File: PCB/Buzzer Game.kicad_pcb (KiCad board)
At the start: 2 copper layers, 50 x 50 mm, 23 parts, among them J1 Conn_01x02, Q1 BC547, Q2 BC547, U1 74LS373

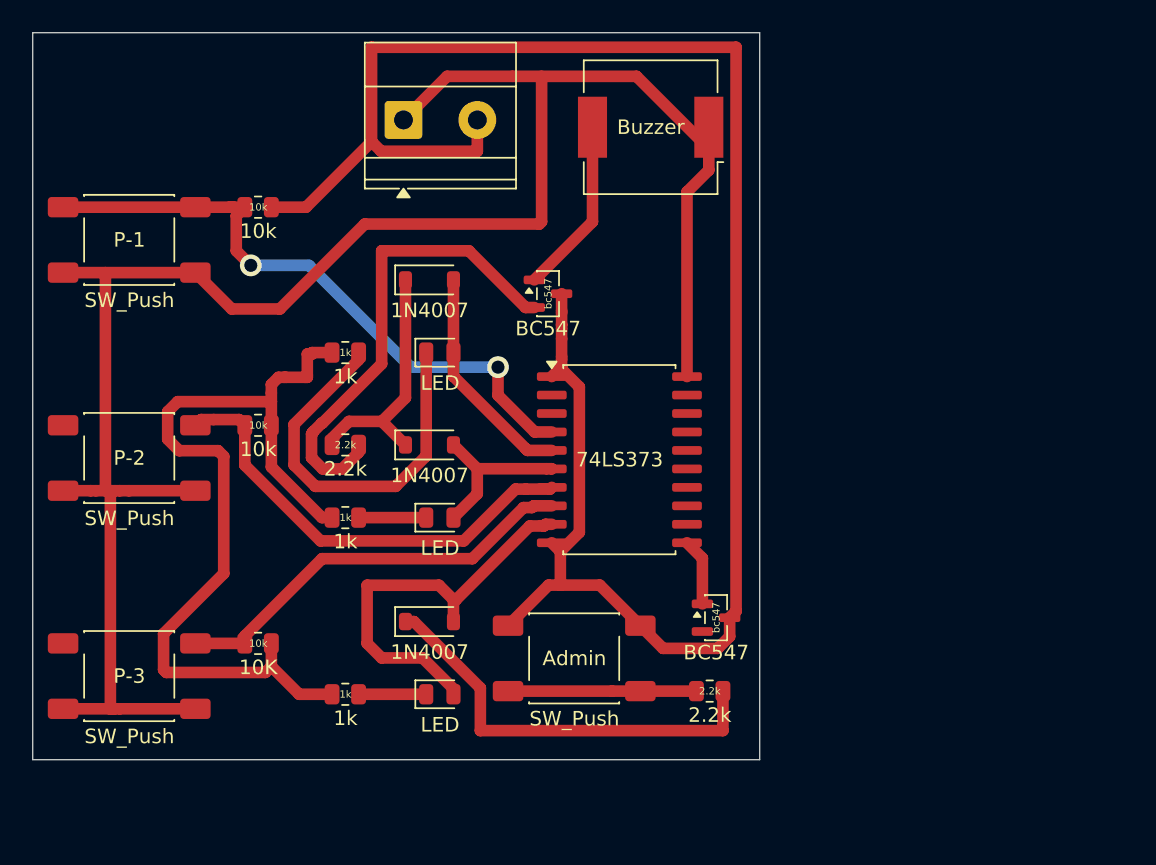
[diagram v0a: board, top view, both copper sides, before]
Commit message: .
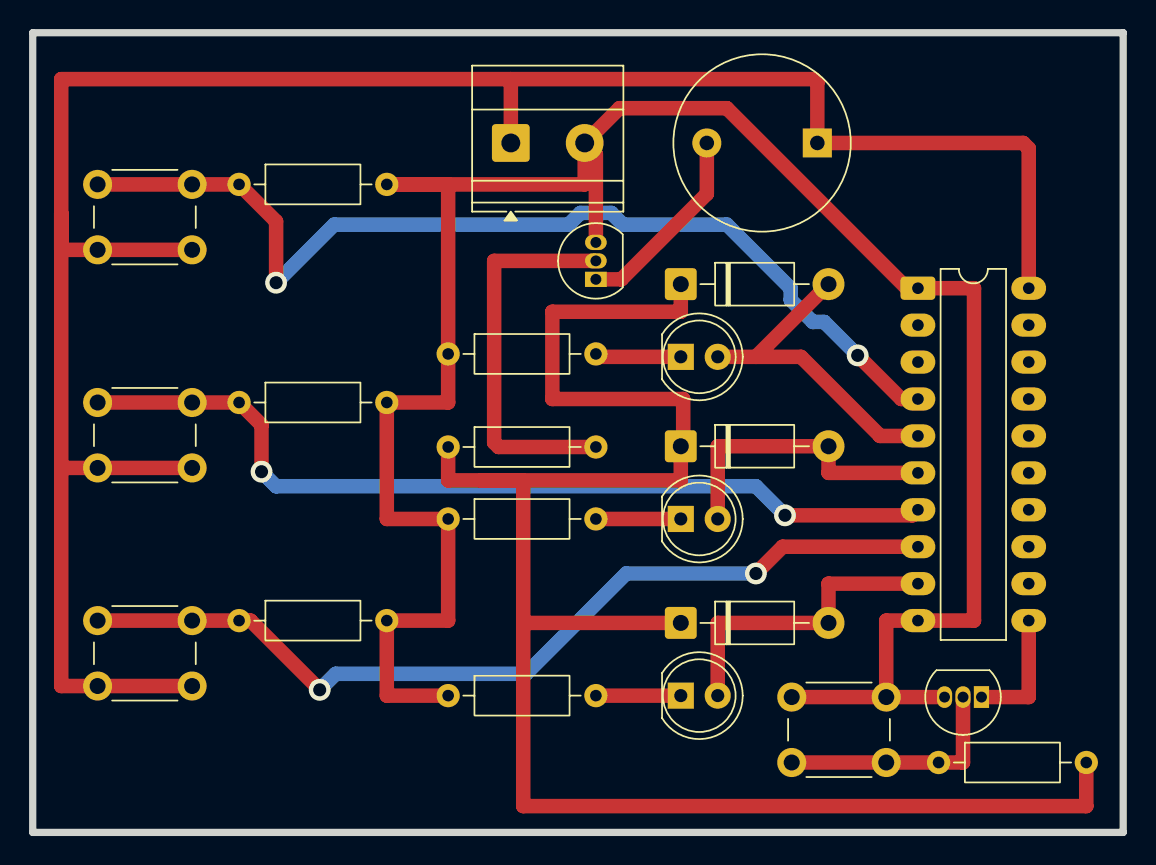
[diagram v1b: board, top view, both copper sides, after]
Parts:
- Admin1, P-1, P-2, P-3: footprint Button_Switch_SMD:SW_Push_1P1T_NO_E-Switch_TL3301NxxxxxG -> Button_Switch_THT:SW_PUSH_6mm
- BZ1: footprint Buzzer_Beeper:Buzzer_CUI_CPT-9019S-SMT -> Buzzer_Beeper:Buzzer_12x9.5RM7.6
- D1, D2, D3: footprint Diode_SMD:D_SOD-123 -> Diode_THT:D_DO-41_SOD81_P10.16mm_Horizontal
- D4, D5, D6: footprint LED_SMD:LED_0805_2012Metric -> LED_THT:LED_D5.0mm
- Q1, Q2: footprint Package_TO_SOT_SMD:SOT-23 -> Package_TO_SOT_THT:TO-92_Inline
- R1, R2: value 10k -> R; footprint Resistor_SMD:R_0805_2012Metric -> Resistor_THT:R_Axial_DIN0207_L6.3mm_D2.5mm_P10.16mm_Horizontal
- R3: value 10K -> R; footprint Resistor_SMD:R_0805_2012Metric -> Resistor_THT:R_Axial_DIN0207_L6.3mm_D2.5mm_P10.16mm_Horizontal
- R4, R8: value 2.2k -> R; footprint Resistor_SMD:R_0805_2012Metric -> Resistor_THT:R_Axial_DIN0207_L6.3mm_D2.5mm_P10.16mm_Horizontal
- R5, R6, R7: value 1k -> R; footprint Resistor_SMD:R_0805_2012Metric -> Resistor_THT:R_Axial_DIN0207_L6.3mm_D2.5mm_P10.16mm_Horizontal
- U1: footprint Package_SO:SOIC-20W_7.5x12.8mm_P1.27mm -> Package_DIP:DIP-20_W7.62mm_LongPads
- moved U1 23.7 mm to (60.9, 17.6)
- moved Q1 19.1 mm to (65.3, 45.7), turned to 180 degrees
- moved D1 17.3 mm to (44.6, 17.3)
- moved D2 17.3 mm to (44.6, 28.4)
- moved D3 17.3 mm to (44.6, 40.6)
- moved D4 16.6 mm to (44.6, 22.3)
- moved D5 16.6 mm to (44.6, 33.4)
- moved D6 16.6 mm to (44.6, 45.6)
- moved R4 16.5 mm to (62.3, 50.2)
- moved Admin1 15.2 mm to (52.2, 45.7)
- moved BZ1 11.5 mm to (54.0, 7.58)
- moved J1 7.55 mm to (32.9, 7.58)
- moved R8 7.07 mm to (28.6, 28.5)
- moved R5 7.07 mm to (28.6, 22.1)
- moved R6 7.07 mm to (28.6, 33.4)
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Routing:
- net /D-: track 46.4 -> 127.6 mm
- net GND: track 193.7 -> 157.4 mm
- net /S3: track 28.7 -> 62.5 mm, vias 0 -> 2
- net /S2: track 31.3 -> 61.7 mm, vias 0 -> 2
- net /S1: track 43.7 -> 69.4 mm
- net Net-(D4-K): track 27.2 -> 5.92 mm
- net VCC: track 136.7 -> 156.3 mm
- net /O2: track 11.5 -> 20.6 mm
- net /O1: track 15.5 -> 23.1 mm
- net /O3: track 28.4 -> 21.5 mm
- net Net-(Q2-B): track 32.9 -> 26.6 mm
- net /ENG: track 4.64 -> 8.51 mm
- net /B: track 13.0 -> 16.3 mm
- net /B-: track 12.2 -> 13.6 mm
- net Net-(D6-K): track 4.65 -> 5.84 mm
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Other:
- board size 50 x 50 mm -> 75 x 55 mm
- rule pad_to_mask_clearance: 0 -> 0.2
- board text removed: "10K"
- board text removed: "10k"
- board text removed: "1N4007"
- board text removed: "1k"
- board text removed: "2.2k"
- board text removed: "74LS373"
- board text removed: "Admin"
- board text removed: "BC547"
- board text removed: "Buzzer"
- board text removed: "LED"
- board text removed: "P-1"
- board text removed: "P-2"
- board text removed: "P-3"
- board text removed: "SW_Push"
- board text removed: "bc547"
